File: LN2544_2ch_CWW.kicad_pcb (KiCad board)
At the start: 2 copper layers, 22 x 28 mm, 44 parts, among them P1 Vin, P2 LED, P3 DIM, P4 NTC, U1 LN2544, U2 LN2544

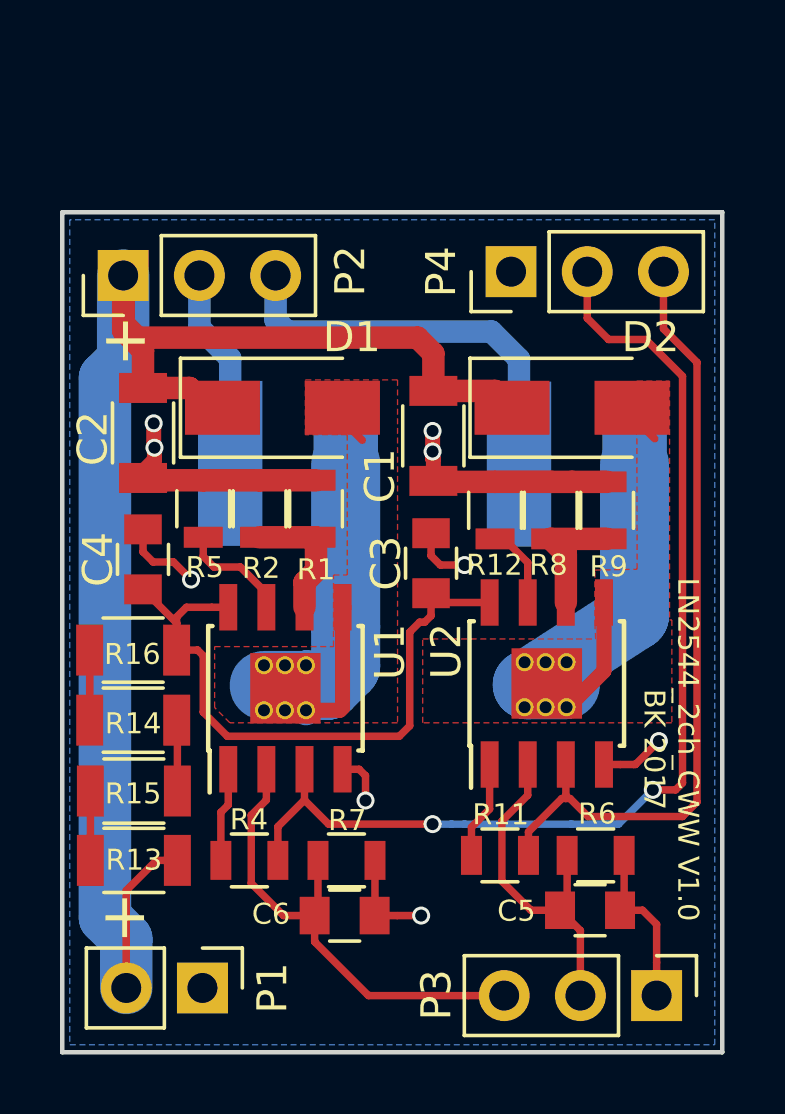
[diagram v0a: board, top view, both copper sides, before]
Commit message: V1.1 Update
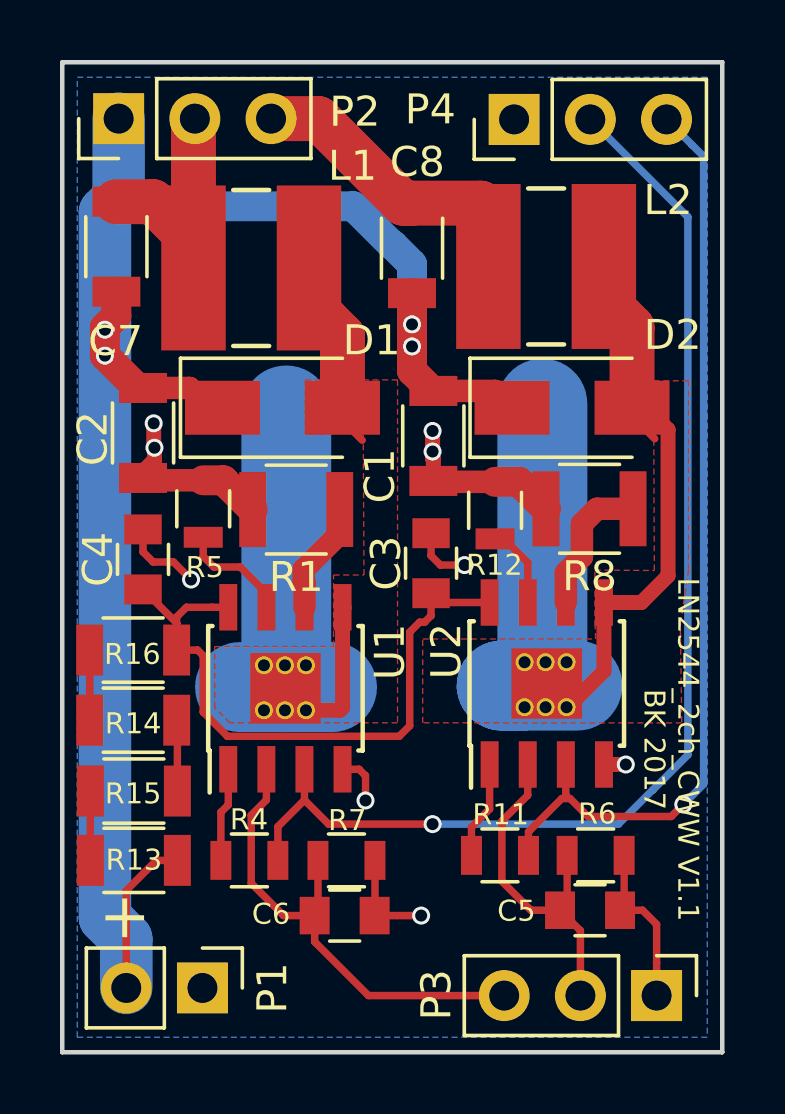
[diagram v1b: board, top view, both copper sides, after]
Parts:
- removed R2: R_CS12, Resistors_SMD:R_0805
- removed R9: R_CS22, Resistors_SMD:R_0805
- added C7: 1u/50V, Capacitors_SMD:C_1206, F.Cu at (101.8, 101.1)
- added C8: 1u/50V, Capacitors_SMD:C_1206, F.Cu at (111.7, 101.2)
- L1, L2: value 39uH -> 68uH; moved to F.Cu
- R1: value R_CS11 -> 1R5; footprint Resistors_SMD:R_0805 -> Resistors_SMD:R_1210
- R11: value RNTC2 -> 24k
- R12: value RO2 -> 24k
- R4: value RNTC1 -> 24k
- R5: value RO1 -> 24k
- R6, R7: value 10K -> 62k
- R8: value R_CS21 -> 1R5; footprint Resistors_SMD:R_0805 -> Resistors_SMD:R_1210
- moved REF*** 14.2 mm to (111.0, 102.7)
- moved REF*** 7.00 mm to (110.9, 109.4)
- moved L2 6.67 mm to (116.1, 101.8)
- moved L1 6.63 mm to (106.3, 101.9)
- moved P2 5.23 mm to (101.9, 96.9)
- moved P4 5.08 mm to (115.1, 96.9)
- moved R8 1.30 mm to (117.6, 109.9), turned to 180 degrees
- moved R1 0.66 mm to (107.8, 109.9), turned to 180 degrees
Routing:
- net /DRAIN2: track 27.8 -> 38.9 mm
- net VCC: track 53.3 -> 64.0 mm, vias 0 -> 4
- net /DRAIN1: track 22.9 -> 29.9 mm
- net /NTC2: track 27.3 -> 32.3 mm, vias 0 -> 1
- net GND: track 33.2 -> 28.4 mm
- net /NTC1: track 36.0 -> 40.0 mm, vias 2 -> 1
- net /LEDN2: track 13.6 -> 10.4 mm
- net /LEDN1: track 6.69 -> 9.35 mm
- net /CS1: track 4.37 -> 3.77 mm
- net /CS2: track 4.21 -> 4.76 mm
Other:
- board size 22 x 28 mm -> 22 x 33 mm
- board text added: "LN2544_2ch_CWW V1.1"
- board text added: "LN2544_2ch_CWW V1.1 BK 2017"
- board text removed: "LN2544_2ch_CWW V1.0"
- board text removed: "LN2544_2ch_CWW V1.0 BK 2017"
